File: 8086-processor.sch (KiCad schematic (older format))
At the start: 20 parts, among them SW25 SW_Push, U18 8086_Min_Mode, U19 74LS374, U20 74LS244, U21 74LS374, U22 74LS374, U23 74LS245, U24 74LS245

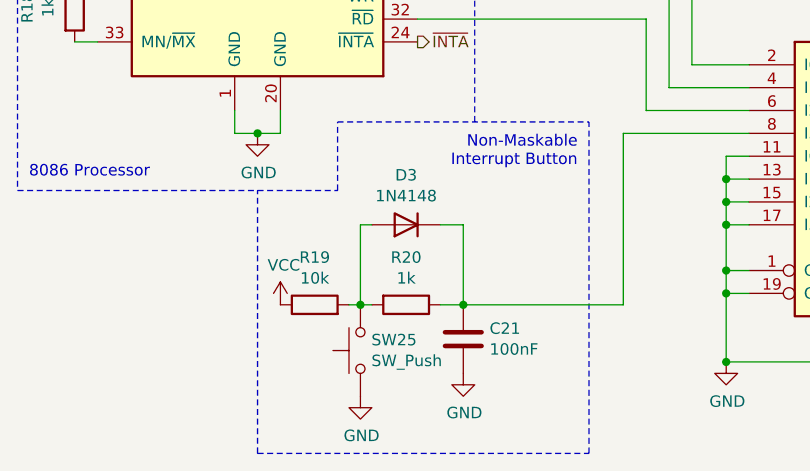
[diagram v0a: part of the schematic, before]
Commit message: assign footprints and edits
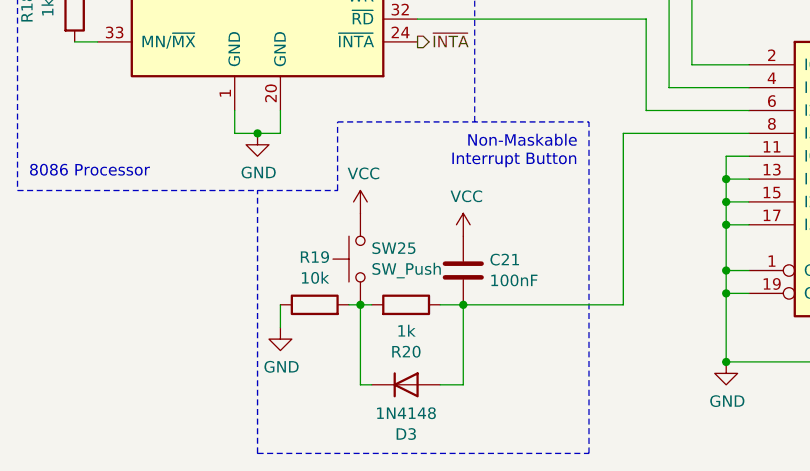
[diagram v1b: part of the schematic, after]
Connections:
- net GND: now also R19.1; no longer C21.2, SW25.1
- net VCC: now also C21.1, SW25.2; no longer R19.1
- net at R20.1, U20.8 (I3a): now also C21.2, D3.2 (A); no longer C21.1, D3.1 (K)
- net at R19.2, R20.2: now also D3.1 (K), SW25.1; no longer D3.2 (A), SW25.2
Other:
- moved on the sheet: C21, D3, SW25
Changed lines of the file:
@@
 	2300 7000 2250 7000
-$Comp
-L power:GND #PWR0191
-U 1 1 627AC8BB
-P 2700 7300
-F 0 "#PWR0191" H 2700 7050 50  0001 C CNN
-F 1 "GND" H 2705 7127 50  0000 C CNN
-F 2 "" H 2700 7300 50  0001 C CNN
-F 3 "" H 2700 7300 50  0001 C CNN
-	1    2700 7300
-	1    0    0    -1
-$EndComp
 $Comp
 L Device:R R20
@@
 F 3 "~" H 2450 7000 50  0001 C CNN
 	1    2450 7000
-	0    1    1    0
+	0    1    -1   0
 $EndComp
 $Comp
 L power:VCC #PWR0192
 U 1 1 6278DB4C
-P 1900 7000
-F 0 "#PWR0192" H 1900 6850 50  0001 C CNN
-F 1 "VCC" H 1915 7173 50  0000 C CNN
-F 2 "" H 1900 7000 50  0001 C CNN
-F 3 "" H 1900 7000 50  0001 C CNN
-	1    1900 7000
+P 2700 6700
+F 0 "#PWR0192" H 2700 6550 50  0001 C CNN
+F 1 "VCC" H 2715 6873 50  0000 C CNN
+F 2 "" H 2700 6700 50  0001 C CNN
+F 3 "" H 2700 6700 50  0001 C CNN
+	1    2700 6700
 	1    0    0    -1
 $EndComp
@@
 L Device:C C21
 U 1 1 6277FDCA
-P 2700 7150
-F 0 "C21" H 2815 7196 50  0000 L CNN
-F 1 "100nF" H 2815 7105 50  0000 L CNN
-F 2 "Capacitor_THT:C_Rect_L4.0mm_W2.5mm_P2.50mm" H 2738 7000 50  0001 C CNN
-F 3 "~" H 2700 7150 50  0001 C CNN
-	1    2700 7150
+P 2700 6850
+F 0 "C21" H 2815 6896 50  0000 L CNN
+F 1 "100nF" H 2815 6805 50  0000 L CNN
+F 2 "Capacitor_THT:C_Rect_L4.0mm_W2.5mm_P2.50mm" H 2738 6700 50  0001 C CNN
+F 3 "~" H 2700 6850 50  0001 C CNN
+	1    2700 6850
 	1    0    0    -1
 $EndComp
@@
 L Switch:SW_Push SW25
 U 1 1 626B0BE8
-P 2250 7200
-F 0 "SW25" V 2296 7152 50  0000 R CNN
-F 1 "SW_Push" V 2205 7152 50  0000 R CNN
-F 2 "Button_Switch_Keyboard:SW_Cherry_MX_1.00u_PCB" H 2250 7400 50  0001 C CNN
-F 3 "~" H 2250 7400 50  0001 C CNN
-	1    2250 7200
+P 2250 6800
+F 0 "SW25" V 2296 6752 50  0000 R CNN
+F 1 "SW_Push" V 2205 6752 50  0000 R CNN
+F 2 "Button_Switch_Keyboard:SW_Cherry_MX_1.00u_PCB" H 2250 7000 50  0001 C CNN
+F 3 "~" H 2250 7000 50  0001 C CNN
+	1    2250 6800
 	0    -1   -1   0
 $EndComp
@@
 L power:GND #PWR0193
 U 1 1 6233B1ED
-P 2250 7400
-F 0 "#PWR0193" H 2250 7150 50  0001 C CNN
-F 1 "GND" H 2255 7227 50  0000 C CNN
-F 2 "" H 2250 7400 50  0001 C CNN
-F 3 "" H 2250 7400 50  0001 C CNN
-	1    2250 7400
+P 1900 7100
+F 0 "#PWR0193" H 1900 6850 50  0001 C CNN
+F 1 "GND" H 1905 6927 50  0000 C CNN
+F 2 "" H 1900 7100 50  0001 C CNN
+F 3 "" H 1900 7100 50  0001 C CNN
+	1    1900 7100
 	1    0    0    -1
 $EndComp
@@
 L Diode:1N4148 D?
 U 1 1 61F82EF7
-P 2450 6650
+P 2450 7350
 AR Path="/61CB92C1/61F82EF7" Ref="D?"  Part="1"
 AR Path="/6190420C/61F82EF7" Ref="D3"  Part="1"
-F 0 "D3" H 2450 6433 50  0000 C CNN
-F 1 "1N4148" H 2450 6524 50  0000 C CNN
-F 2 "Diode_THT:D_DO-35_SOD27_P7.62mm_Horizontal" H 2450 6475 50  0001 C CNN
-F 3 "https://assets.nexperia.com/documents/data-sheet/1N4148_1N4448.pdf" H 2450 6650 50  0001 C CNN
-	1    2450 6650
-	-1   0    0    1
+F 0 "D3" H 2450 7133 50  0000 C CNN
+F 1 "1N4148" H 2450 7224 50  0000 C CNN
+F 2 "Diode_THT:D_DO-35_SOD27_P7.62mm_Horizontal" H 2450 7175 50  0001 C CNN
+F 3 "https://assets.nexperia.com/documents/data-sheet/1N4148_1N4448.pdf" H 2450 7350 50  0001 C CNN
+	1    2450 7350
+	1    0    0    -1
 $EndComp
 Wire Notes Line
@@
 Wire Notes Line
 	3250 7650 3250 6200
-Wire Wire Line
-	2600 6650 2700 6650
-Wire Wire Line
-	2300 6650 2250 6650
-Wire Wire Line
-	2250 6650 2250 7000
-Wire Wire Line
-	2700 6650 2700 7000
 Wire Wire Line
 	1100 4050 1000 4050
@@
 	1000 4850 1000 4750
 NoConn ~ 1100 4550
+$Comp
+L power:VCC #PWR04
+U 1 1 61B699AA
+P 2250 6600
+F 0 "#PWR04" H 2250 6450 50  0001 C CNN
+F 1 "VCC" H 2265 6773 50  0000 C CNN
+F 2 "" H 2250 6600 50  0001 C CNN
+F 3 "" H 2250 6600 50  0001 C CNN
+	1    2250 6600
+	1    0    0    -1
+$EndComp
+Wire Wire Line
+	2700 7000 2700 7350
+Wire Wire Line
+	2700 7350 2600 7350
+Wire Wire Line
+	2250 7000 2250 7350
+Wire Wire Line
+	2250 7350 2300 7350
+Wire Wire Line
+	1900 7100 1900 7000
 Wire Bus Line
 	9350 3100 9350 5600
